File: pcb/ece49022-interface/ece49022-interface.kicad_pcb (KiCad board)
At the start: 4 copper layers, 80 x 90 mm, 38 parts, among them J1 Conn_01x03_Pin, J2 Conn_01x05_Pin, J3 Conn_01x04_Pin, J4 Conn_01x04_Pin, J5 Conn_01x02_Pin, J6 Conn_01x02_Pin, Q1 KSC1815, U4 NCP1117-3.3_SOT223, U5 TPS54202DDCT

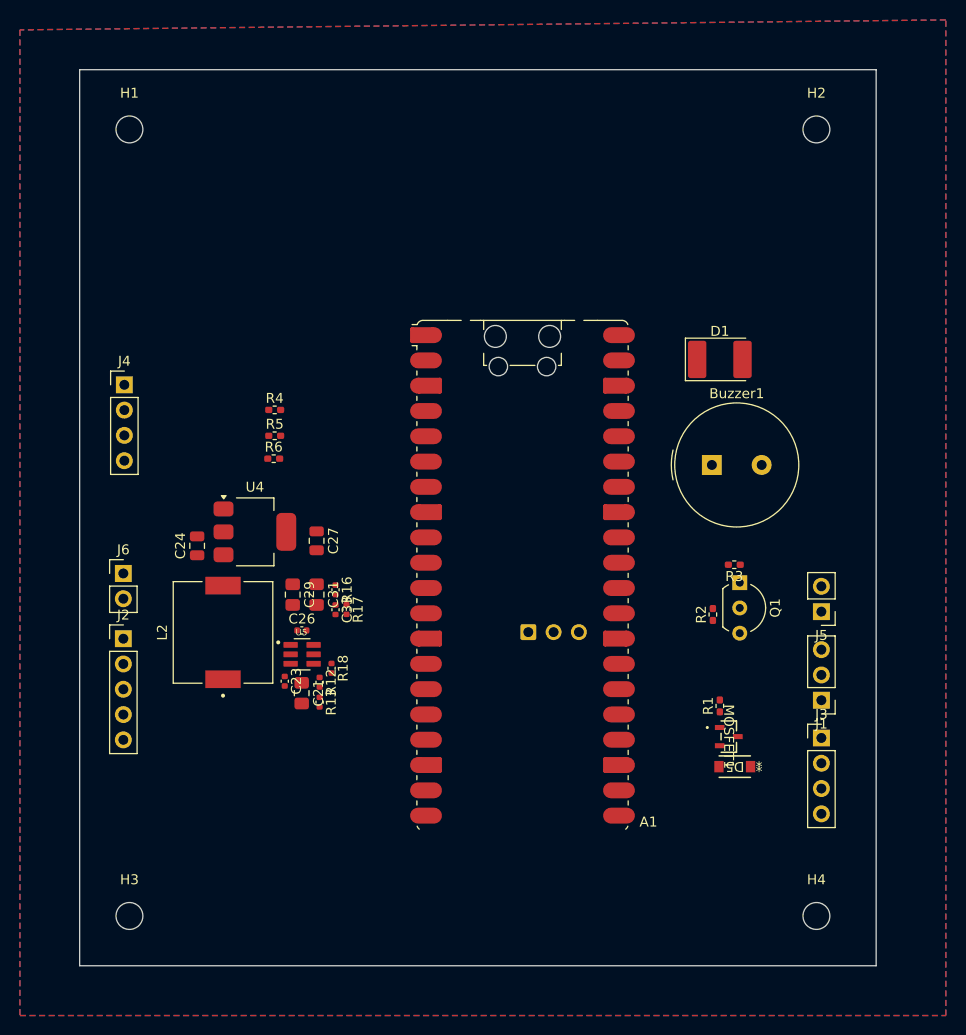
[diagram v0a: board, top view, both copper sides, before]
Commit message: final layout i think
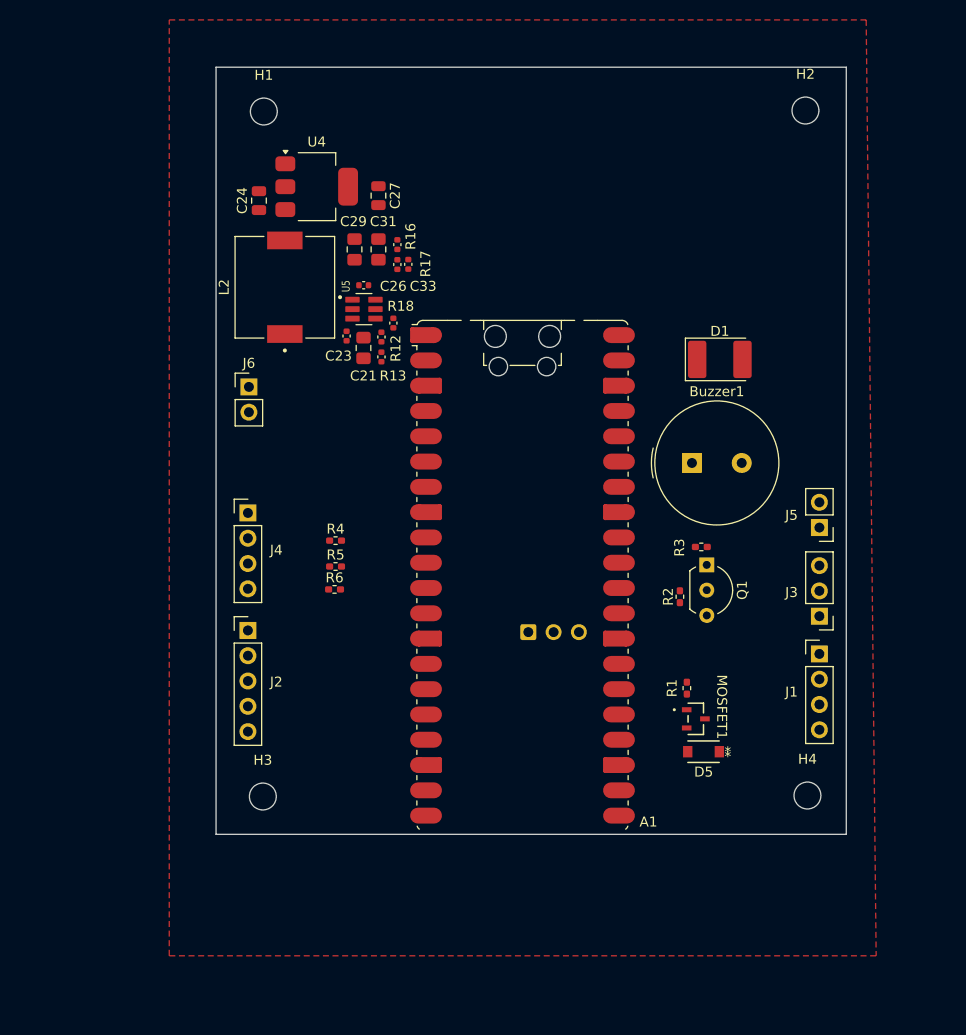
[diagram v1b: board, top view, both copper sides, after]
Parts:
- moved C21 35.2 mm to (141.5, 75.0)
- moved C23 35.2 mm to (139.8, 73.8)
- moved C29 35.2 mm to (140.6, 65.0)
- moved C31 35.2 mm to (143.0, 65.0)
- moved C33 35.2 mm to (144.9, 66.6)
- moved L2 35.2 mm to (133.6, 68.8)
- moved R12 35.2 mm to (143.3, 73.8)
- moved R13 35.2 mm to (143.3, 75.8)
- moved R16 35.2 mm to (144.9, 64.6)
- moved R17 35.2 mm to (146.0, 66.5)
- moved R18 35.2 mm to (144.5, 72.5)
- moved U4 35.2 mm to (136.8, 58.8)
- moved U5 35.2 mm to (141.6, 71.0)
- moved C24 35.2 mm to (131.0, 60.1)
- moved C27 35.2 mm to (143.0, 59.6)
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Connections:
- A1 pad 10: unconnected-(A1-GPIO7-Pad10) -> Net-(A1-GPIO7)
- A1 pad 11: unconnected-(A1-GPIO8-Pad11) -> Net-(A1-GPIO8)
- A1 pad 4: Net-(A1-GPIO2) -> unconnected-(A1-GPIO2-Pad4)
- A1 pad 5: Net-(A1-GPIO3) -> unconnected-(A1-GPIO3-Pad5)
- A1 pad 6: Net-(A1-GPIO4) -> unconnected-(A1-GPIO4-Pad6)
- A1 pad 9: unconnected-(A1-GPIO6-Pad9) -> Net-(A1-GPIO6)
- R4 pad 2: Net-(A1-GPIO2) -> Net-(A1-GPIO6)
- R5 pad 2: Net-(A1-GPIO3) -> Net-(A1-GPIO7)
- R6 pad 2: Net-(A1-GPIO4) -> Net-(A1-GPIO8)
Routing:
- added copper zone on F.Cu, net +3V3
- removed copper zone on B.Cu, net GND
- removed copper zone on F.Cu, net GND
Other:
- board size 80 x 90 mm -> 63.3 x 77 mm
